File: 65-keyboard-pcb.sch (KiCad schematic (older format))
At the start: 153 parts, among them J1 USB4085-GF-A_REVA, SW1 SW_PUSH, U1 ATMEGA32U4, X1 XTAL_GND

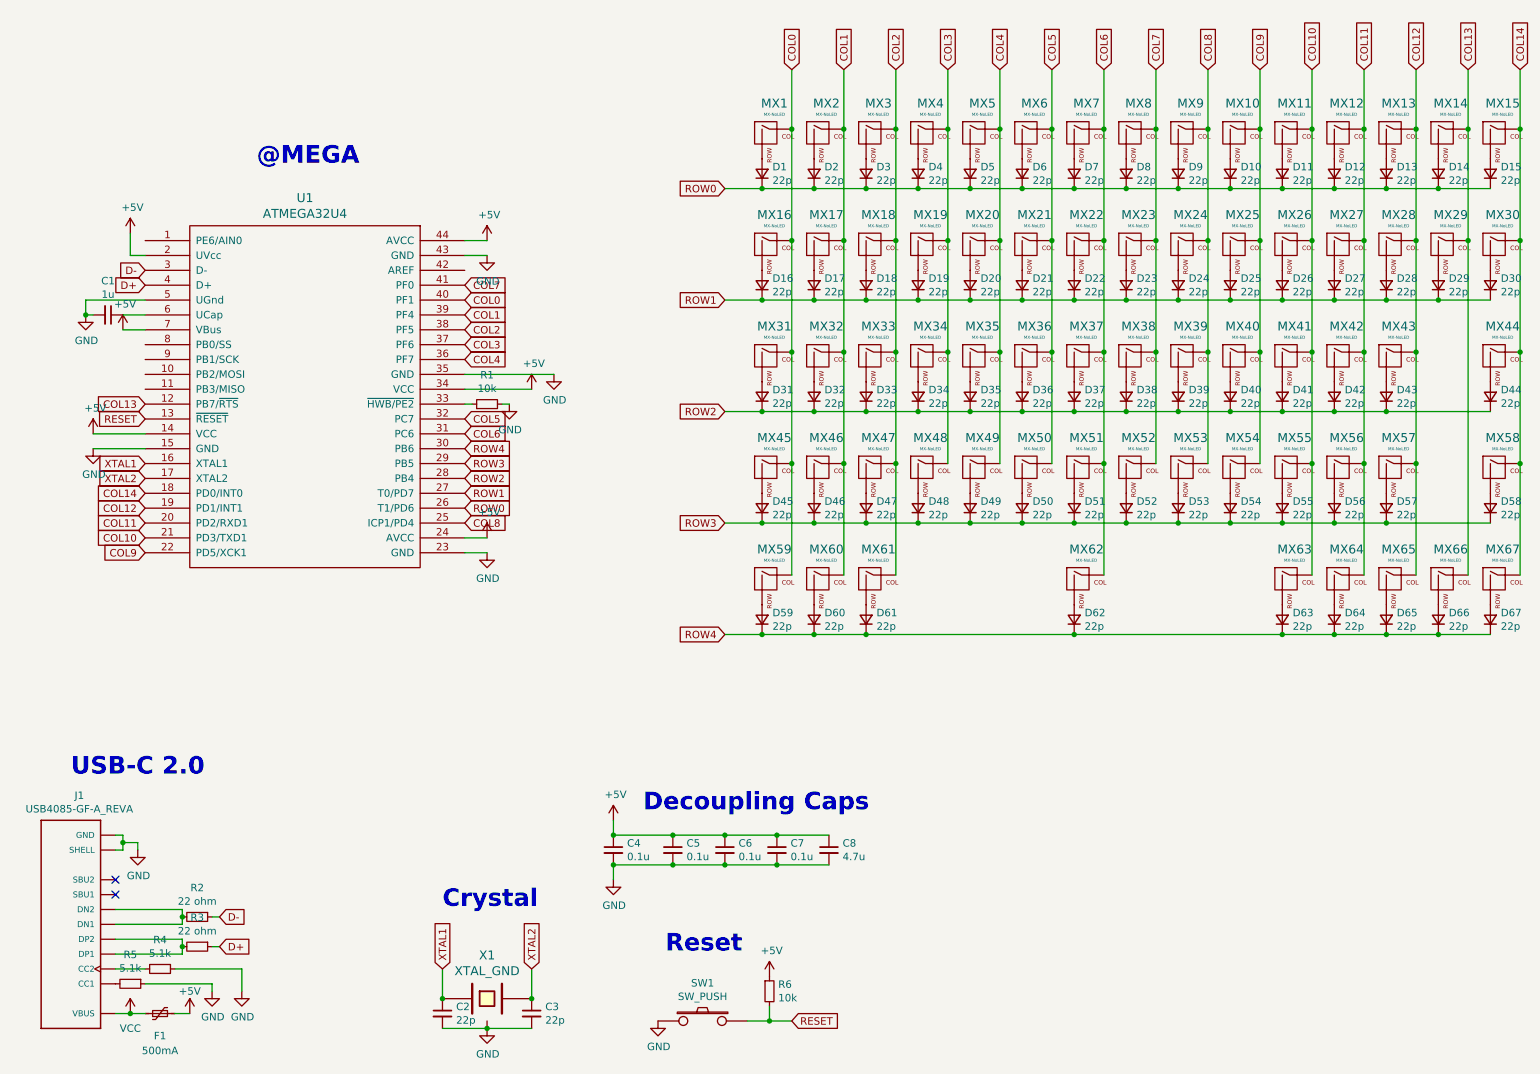
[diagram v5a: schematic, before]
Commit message: PCB
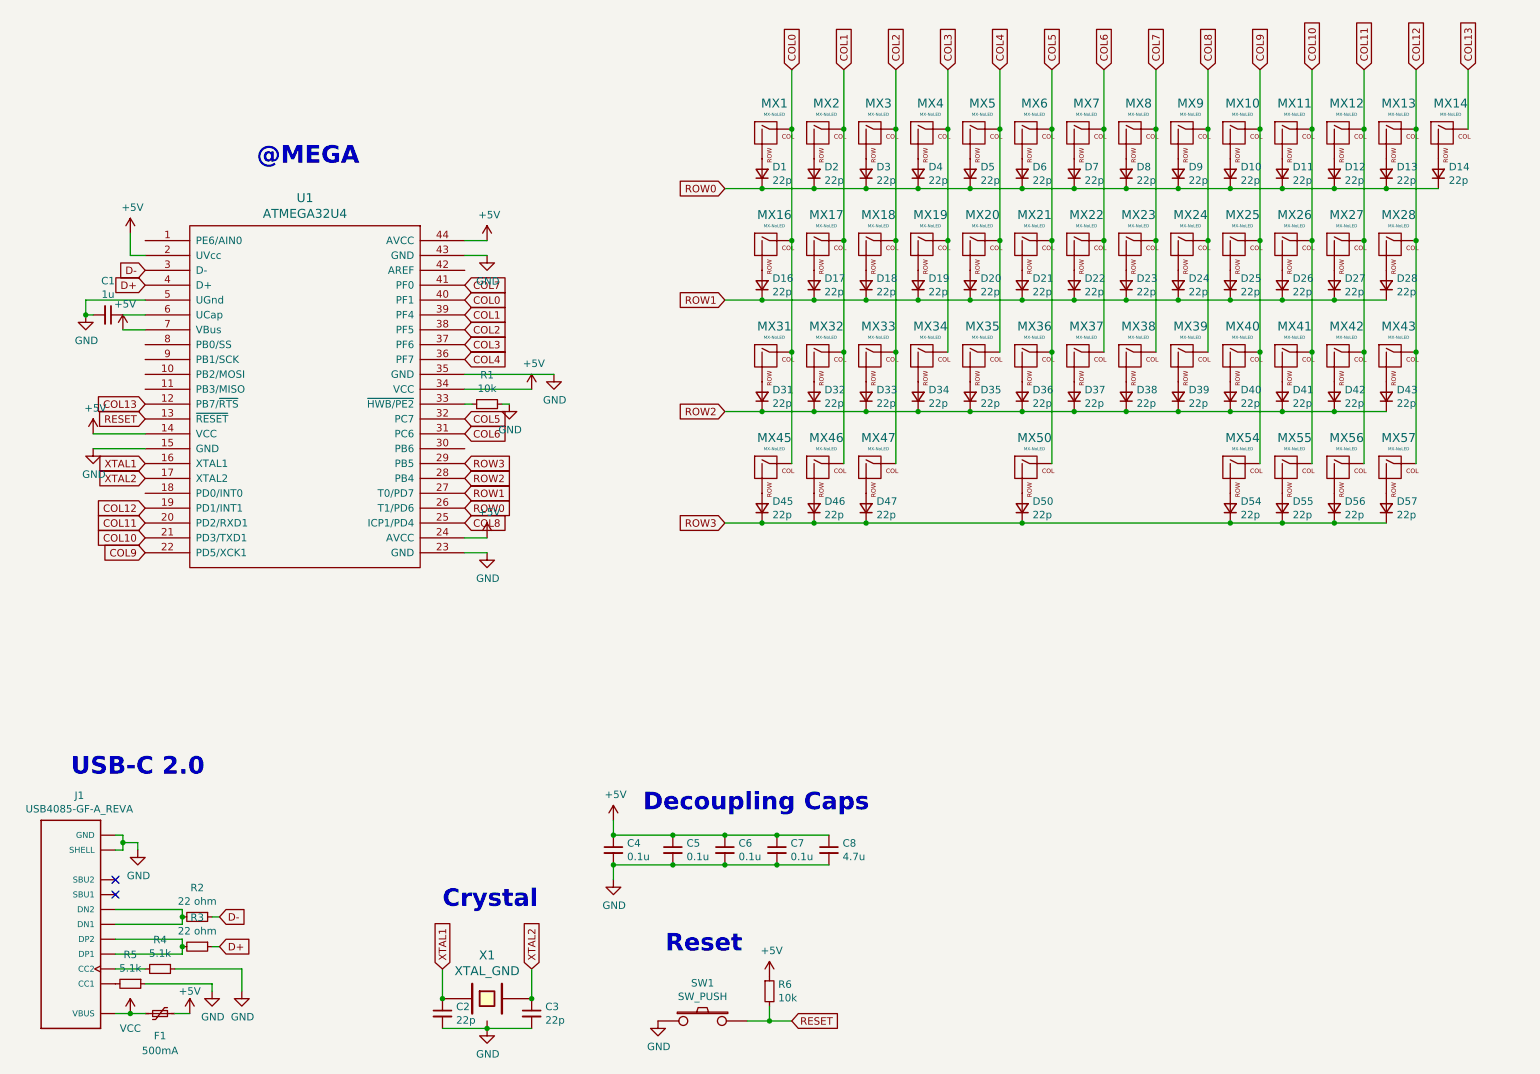
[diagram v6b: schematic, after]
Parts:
- removed D15, D29, D30, D44, D48, D49, D51, D52, D53, D58, D59, D60, D61, D62, D63, D64, D65, D66, D67: 22p, Diode_SMD:D_SOD-123, symbol Device:D_Small
- removed MX15, MX30, MX44, MX48, MX49, MX51, MX52, MX53, MX58, MX64, MX65, MX66, MX67: MX-NoLED, MX_Only:MXOnly-1U-NoLED, symbol MX_Alps_Hybrid:MX-NoLED
- removed MX29: MX-NoLED, MX_Only:MXOnly-1.5U-NoLED, symbol MX_Alps_Hybrid:MX-NoLED
- removed MX59, MX60, MX61, MX63: MX-NoLED, MX_Only:MXOnly-1.25U-NoLED, symbol MX_Alps_Hybrid:MX-NoLED
- removed MX62: MX-NoLED, MX_Only:MXOnly-7U-ReversedStabilizers-NoLED, symbol MX_Alps_Hybrid:MX-NoLED
- MX14: footprint MX_Only:MXOnly-2U-NoLED -> MX_Only:MXOnly-1U-NoLED
- MX16: footprint MX_Only:MXOnly-1.5U-NoLED -> MX_Only:MXOnly-1.25U-NoLED
- MX27: footprint MX_Only:MXOnly-1U-NoLED -> MX_Only:MXOnly-1.75U-NoLED
- MX31: footprint MX_Only:MXOnly-1.25U-NoLED -> MX_Only:MXOnly-1.75U-NoLED
- MX41, MX47, MX54: footprint MX_Only:MXOnly-1U-NoLED -> MX_Only:MXOnly-1.25U-NoLED
- MX43: footprint MX_Only:MXOnly-2.25U-NoLED -> MX_Only:MXOnly-1U-NoLED
- MX45: footprint MX_Only:MXOnly-2.25U-NoLED -> MX_Only:MXOnly-1.25U-NoLED
- MX50: footprint MX_Only:MXOnly-1U-NoLED -> MX_Only:MXOnly-6.25U-ReversedStabilizers-NoLED
- MX56: footprint MX_Only:MXOnly-1.75U-NoLED -> MX_Only:MXOnly-1U-NoLED
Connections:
- net COL14: no longer names the net of U1.18 (PD0/INT0)
- net ROW4: no longer names the net of U1.30 (PB6)
